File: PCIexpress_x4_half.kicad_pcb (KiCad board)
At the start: 4 copper layers, 167.7 x 111.2 mm, 230 parts, among them IC1 TXS0108EPWRG4, IC10 TMDS141RHAR, IC11 TXS0108EPWRG4, IC12 S25FL256LAGMFI001, IC2 TXS0108EPWRG4, IC3 TPS40057PWP, IC4 TPS54620RHLR, IC5 TPS54620RHLR, IC6 MP2359DJ-LF-Z, IC7 MP2315SGJ-Z, IC8 MP2315SGJ-Z, IC9 TMDS141RHAR, J1 PCIexpress_x4, J10 RJ45_RB1-125B8G1A, J11 Conn_02x05_Odd_Even, J12 Conn_01x06_Socket, J2 PCIexpress_bracket, J3 SFP+, J4 SFP+, J5 2-2013289-2, J6 FAN, J7 Jack-DC, J8 HDMI_A_1.4, J9 HDMI_A_1.4, SW1 SW_SPDT, U1 XC7K325T-FFG676, U3 TPS51200DRC, U4 RTL8211EG-VB-CG, U5 SN74LV245ATPWR, U6 TXS0108EPW, U7 TXS0108EPW, Y1 X32-25.000-12-30_30_4085

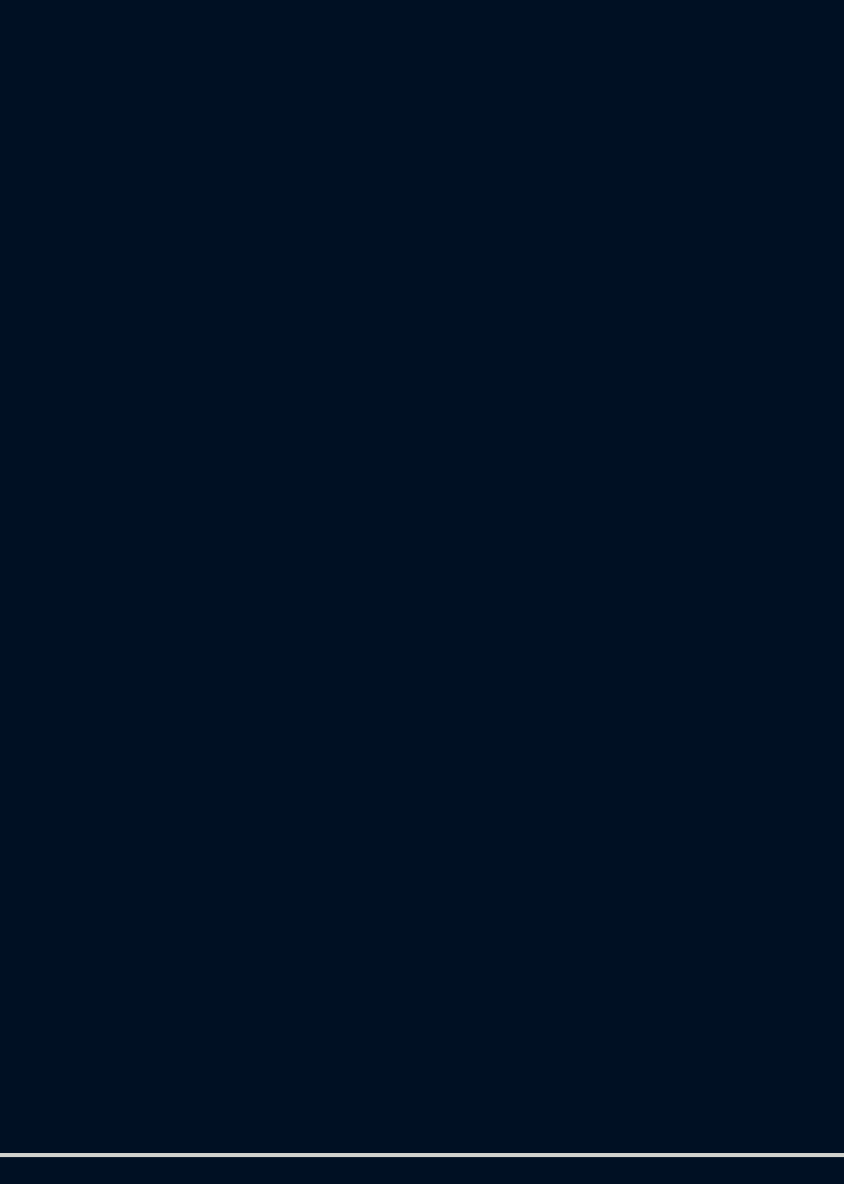
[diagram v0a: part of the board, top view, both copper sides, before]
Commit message: WIP
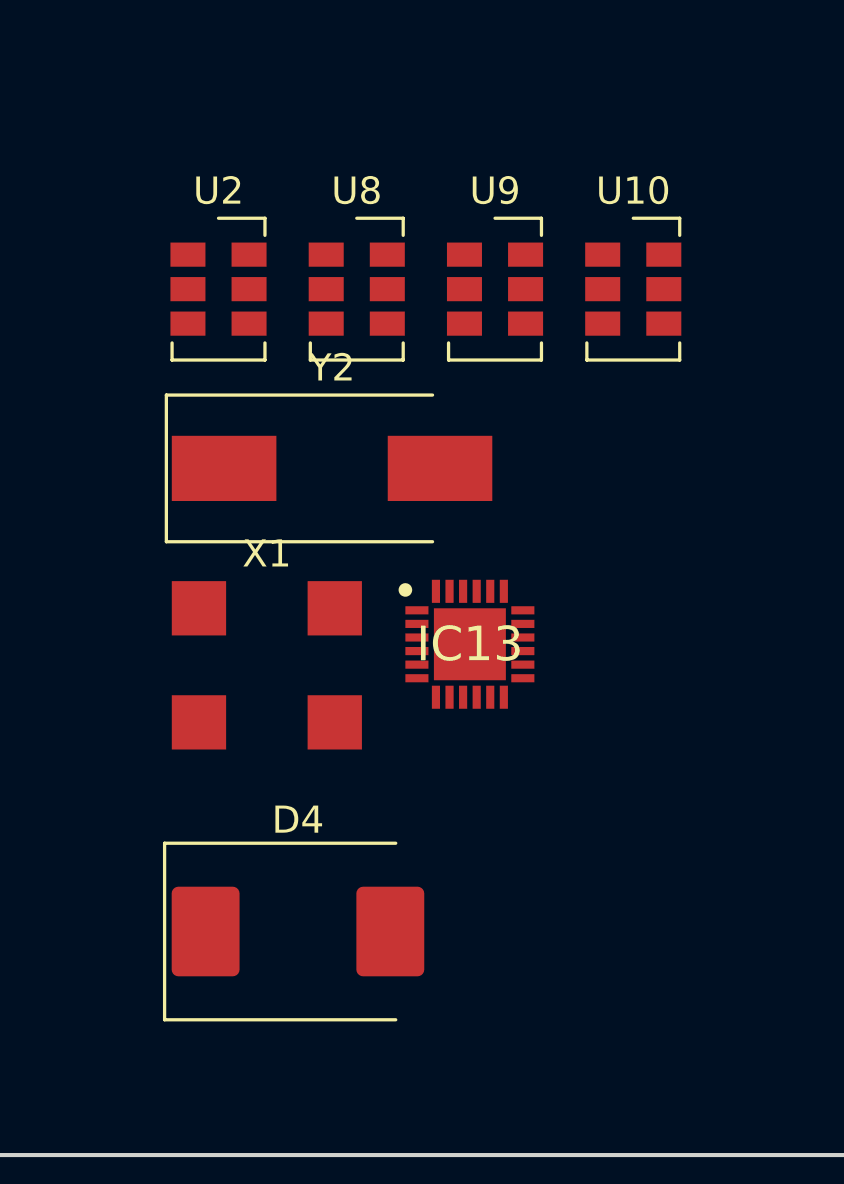
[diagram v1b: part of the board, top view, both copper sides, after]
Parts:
- added D4: B340, Diode_SMD:D_SMC, F.Cu at (129.1, 74.7)
- added IC13: SI5338A-B04911-GM, SamacSys_Parts:QFN50P400X400X90-25N-D, F.Cu at (135.4, 64.2)
- added U10: XUX53, Oscillator:Oscillator_SMD_IDT_JS6-6_5.0x3.2mm_P1.27mm, F.Cu at (141.4, 51.1)
- added U2: XUX53, Oscillator:Oscillator_SMD_IDT_JS6-6_5.0x3.2mm_P1.27mm, F.Cu at (126.2, 51.1)
- added U8: XUX53, Oscillator:Oscillator_SMD_IDT_JS6-6_5.0x3.2mm_P1.27mm, F.Cu at (131.2, 51.1)
- added U9: XUX53, Oscillator:Oscillator_SMD_IDT_JS6-6_5.0x3.2mm_P1.27mm, F.Cu at (136.3, 51.1)
- added X1: XO91, Oscillator:Oscillator_SMD_EuroQuartz_XO91-4Pin_7.0x5.0mm, F.Cu at (127.9, 64.9)
- added Y2: 25M, Crystal:Crystal_SMD_EuroQuartz_MQ2-2Pin_7.0x5.0mm_HandSoldering, F.Cu at (130.3, 57.7)
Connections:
- IC6 pad 1: unconnected-(IC6-BST-Pad1) -> Net-(IC6-BST)
- IC6 pad 2: unconnected-(IC6-GND-Pad2) -> +12V
- IC6 pad 3: unconnected-(IC6-FB-Pad3) -> Net-(IC6-FB)
- IC6 pad 4: unconnected-(IC6-EN-Pad4) -> Net-(IC6-EN)
- IC6 pad 5: unconnected-(IC6-IN-Pad5) -> Net-(IC6-IN)
- IC6 pad 6: unconnected-(IC6-SW-Pad6) -> Net-(D4-K)
- IC8 pad 1: unconnected-(IC8-AAM-Pad1) -> Net-(IC8-AAM)
- IC8 pad 2: unconnected-(IC8-IN-Pad2) -> +12V
- IC8 pad 3: unconnected-(IC8-SW-Pad3) -> Net-(IC8-SW)
- IC8 pad 4: unconnected-(IC8-GND-Pad4) -> +12V
